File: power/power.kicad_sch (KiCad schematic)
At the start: 22 parts, among them J1 XT30, J2 JST Terminal, U1 AP63200WU, U2 AP63200WU

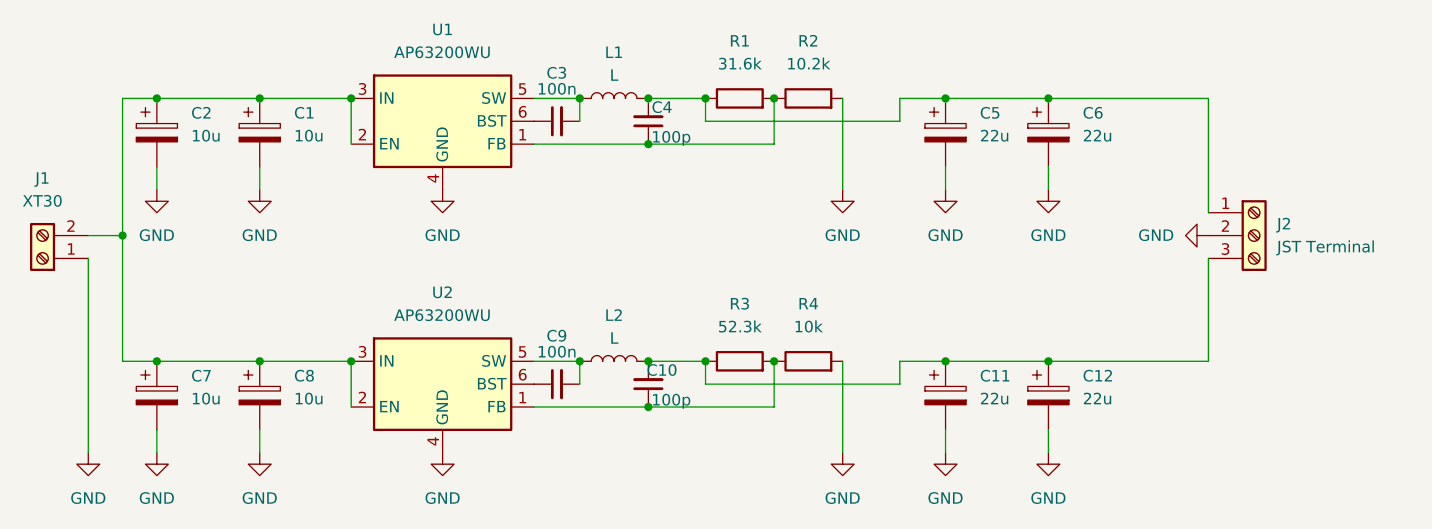
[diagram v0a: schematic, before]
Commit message: refresh
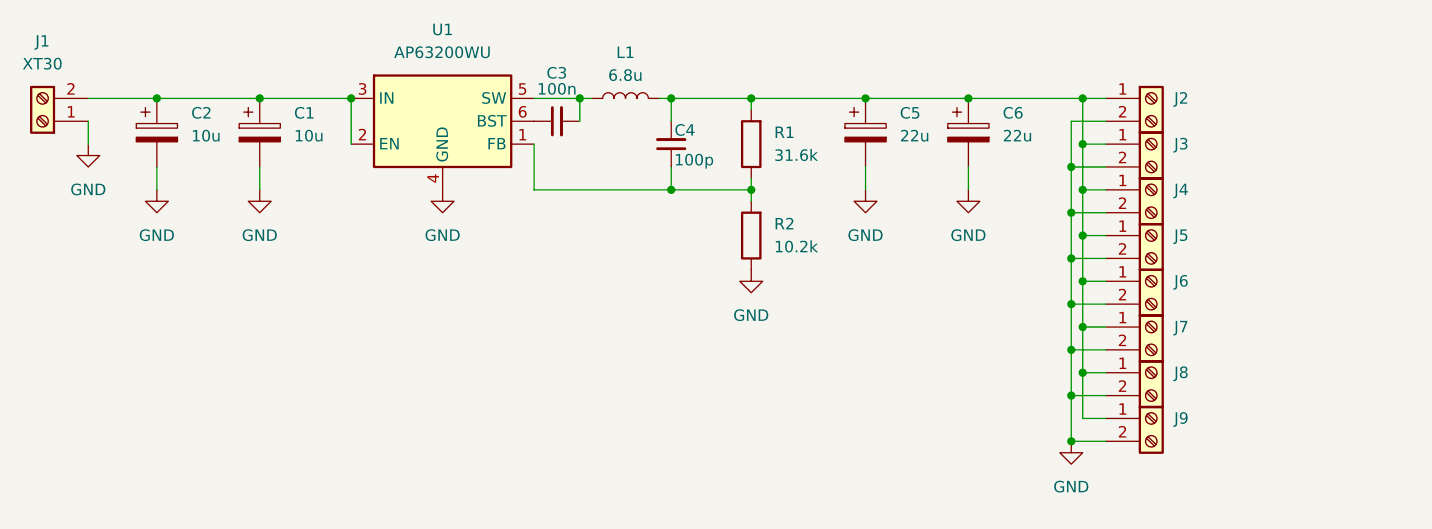
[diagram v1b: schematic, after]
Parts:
- removed C10: 100p, Capacitor_THT:C_Disc_D4.3mm_W1.9mm_P5.00mm, symbol Device:C_Small
- removed C11, C12: 22u, Capacitor_THT:CP_Radial_D5.0mm_P2.50mm, symbol Device:C_Polarized
- removed C7, C8: 10u, Capacitor_THT:CP_Radial_D5.0mm_P2.50mm, symbol Device:C_Polarized
- removed C9: 100n, Capacitor_THT:C_Disc_D4.3mm_W1.9mm_P5.00mm, symbol Device:C_Small
- removed J2: JST Terminal, Connector_JST:JST_PH_B3B-PH-K_1x03_P2.00mm_Vertical, symbol Connector:Screw_Terminal_01x03
- removed L2: L, Inductor_SMD:L_Wuerth_HCI-1890, symbol Device:L
- removed R3: 52.3k, Resistor_THT:R_Axial_DIN0204_L3.6mm_D1.6mm_P2.54mm_Vertical, symbol Device:R
- removed R4: 10k, Resistor_THT:R_Axial_DIN0204_L3.6mm_D1.6mm_P2.54mm_Vertical, symbol Device:R
- removed U2: AP63200WU, Package_TO_SOT_SMD:TSOT-23-6, symbol Regulator_Switching:AP63200WU
- added J2, J3, J4, J5, J6, J7, J8, J9: Screw_Terminal_01x02, Connector_PinHeader_2.54mm:PinHeader_1x02_P2.54mm_Vertical, symbol Connector:Screw_Terminal_01x02
- L1: value L -> 6.8u
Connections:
- net GND: now also R2.1, J2.2 (Pin_2), J3.2 (Pin_2), J4.2 (Pin_2), J5.2 (Pin_2), J6.2 (Pin_2), J7.2 (Pin_2), J8.2 (Pin_2), J9.2 (Pin_2); no longer R2.2
- net at C4.1, U1.1 (FB): now also R1.1, R2.2; no longer R1.2, R2.1
- net at C4.2, C5.1, C6.1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: now also R1.2, J2.1 (Pin_1), J3.1 (Pin_1), J4.1 (Pin_1), J5.1 (Pin_1), J6.1 (Pin_1), J7.1 (Pin_1), J8.1 (Pin_1), J9.1 (Pin_1); no longer R1.1
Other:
- moved on the sheet: C4, C5, C6, J1, L1, R1, R2
